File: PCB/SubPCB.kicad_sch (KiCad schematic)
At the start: 61 parts, among them U10 TLP222A, U11 TLP222A, U12 TLP222A, U13 TLP222A, U14 TLP222A, U15 TLP222A, U16 TLP222A, U17 TLP222A, U18 TLP222A, U2 TLP785, U3 TLP785, U38 MCP2562-E-P, U4 TLP785, U5 TLP785, U6 TLP785, U7 TLP785, U8 TLP785, U9 TLP785

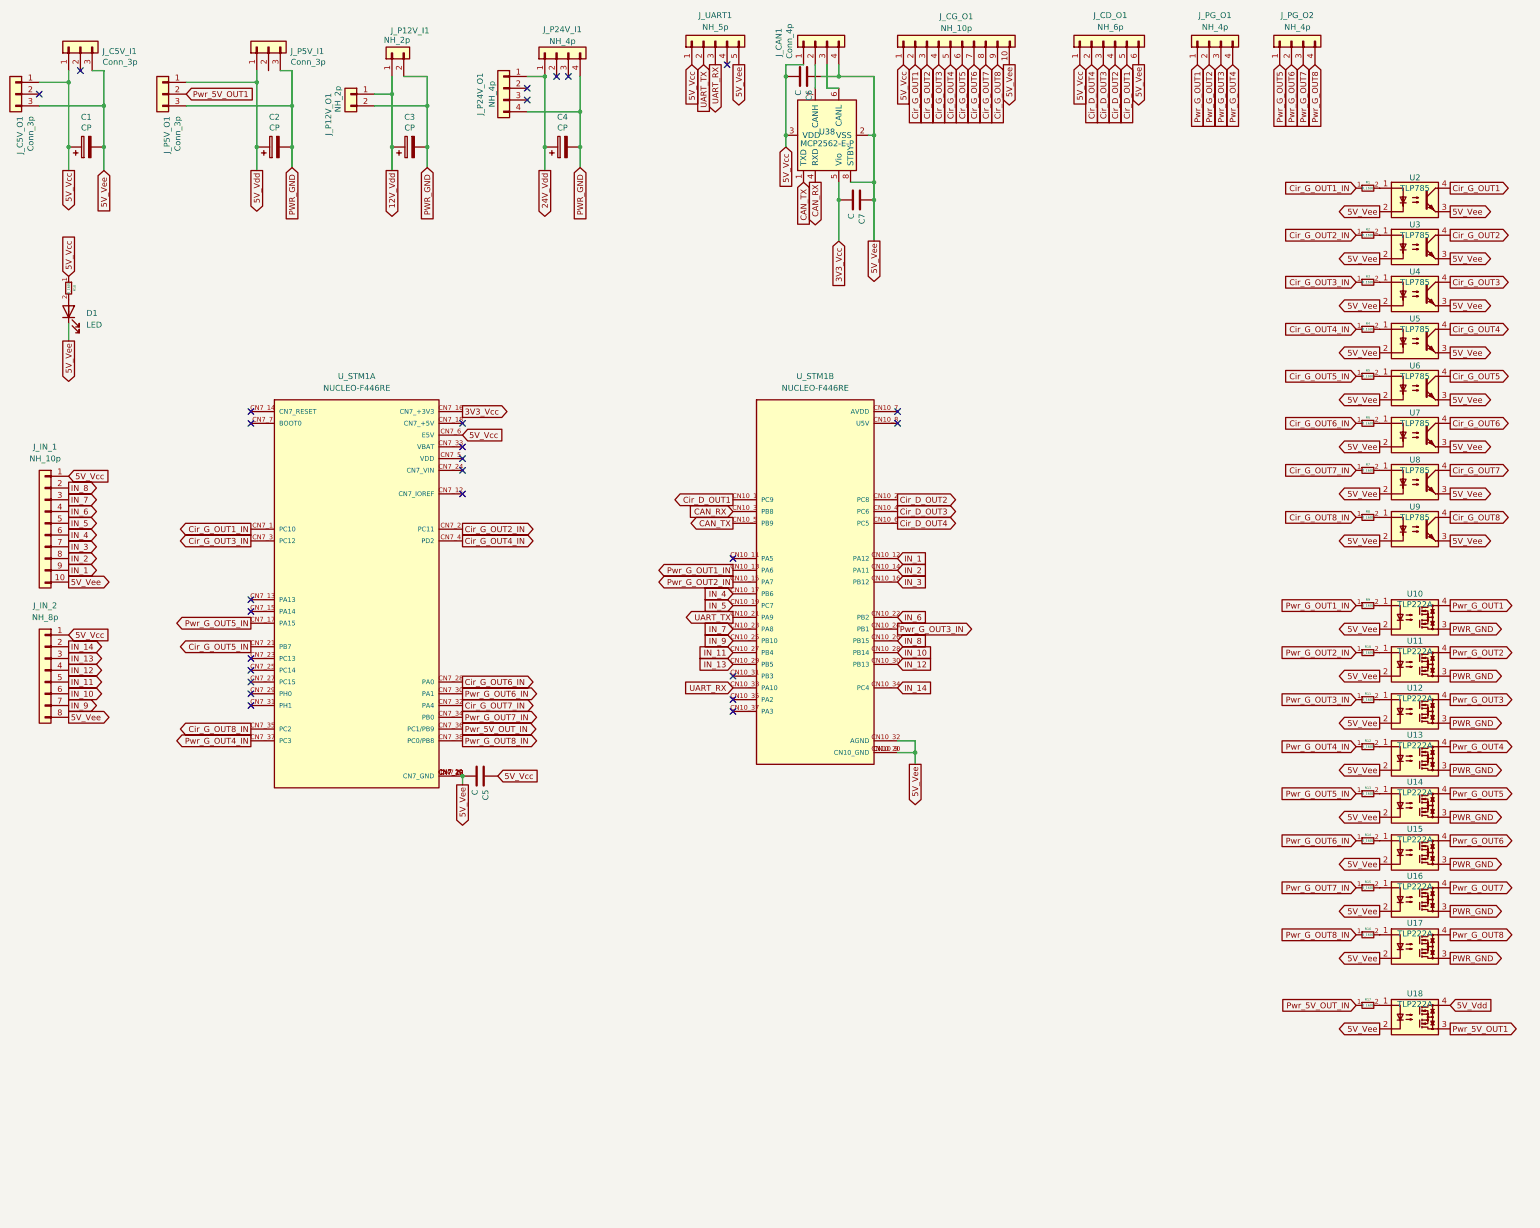
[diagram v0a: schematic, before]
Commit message: add
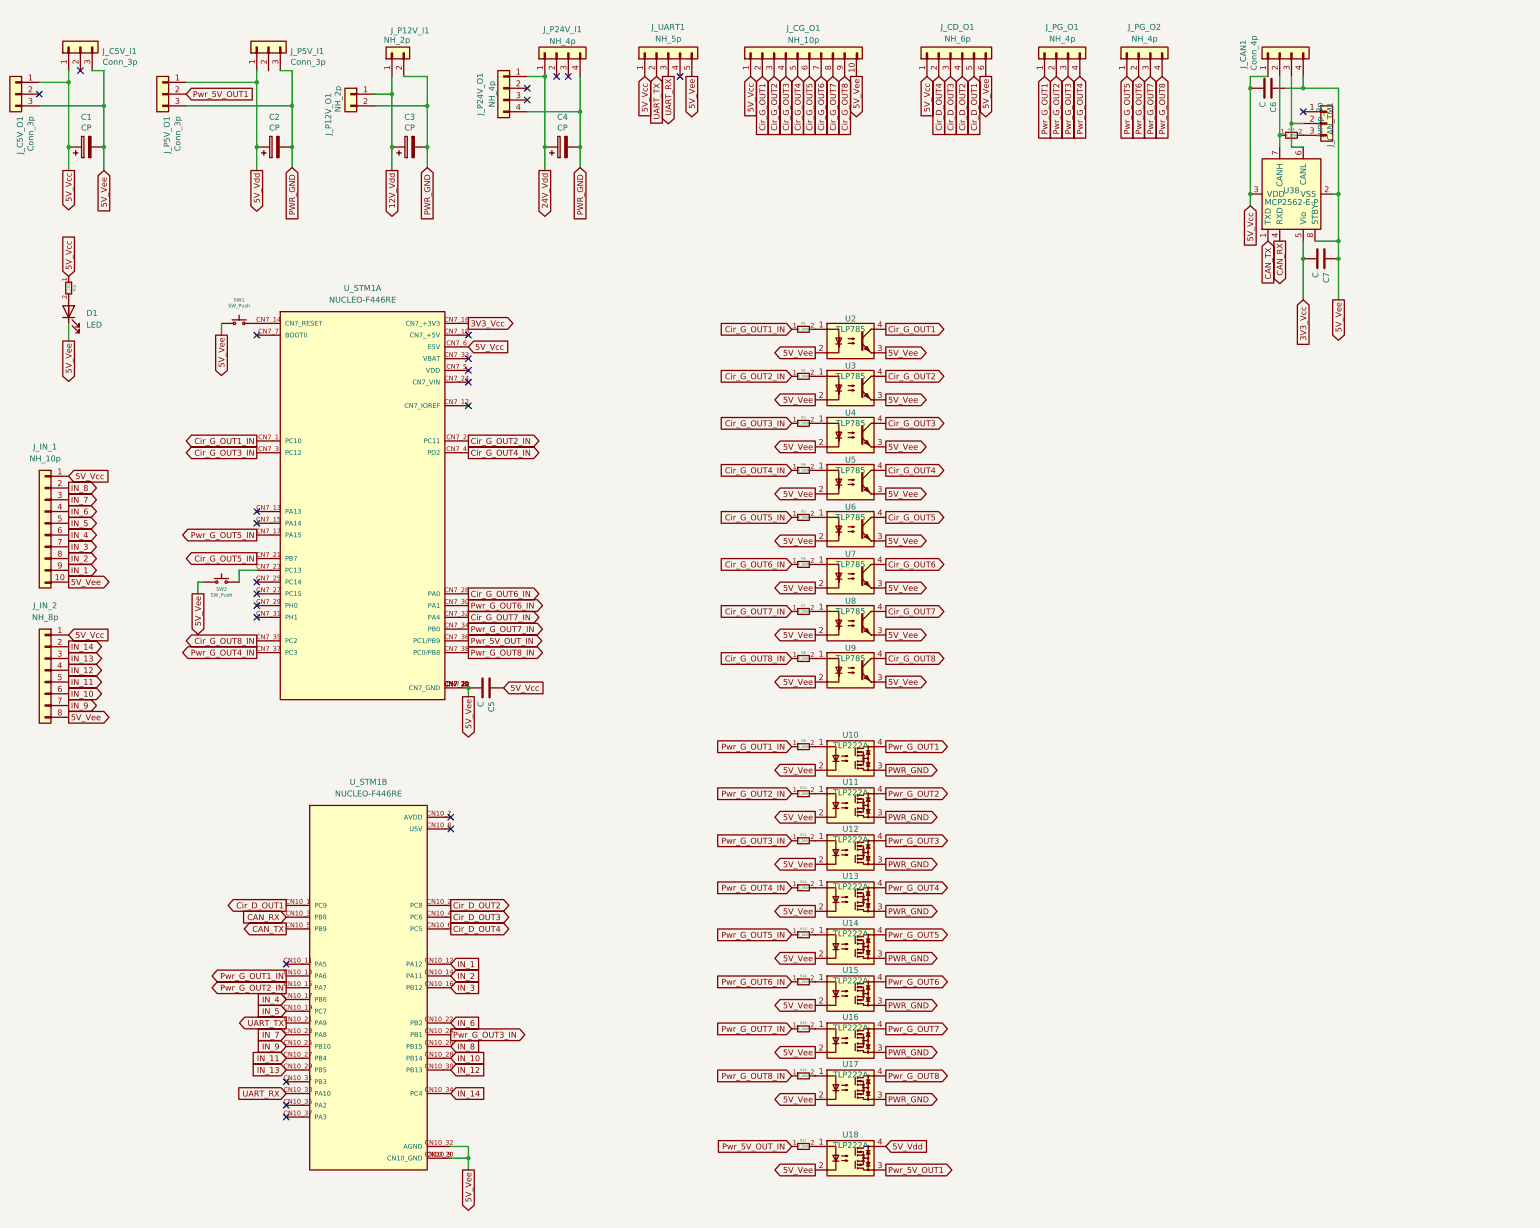
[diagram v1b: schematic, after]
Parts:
- added J_CAN_TM1: Jump_3p, KAZAAAN:Conn_3pin, symbol SubPCB-rescue:Conn_3p-KAZAAAN_Library
- added R19: R_1608, Resistor_SMD:R_0603_1608Metric_Pad0.98x0.95mm_HandSolder, symbol R_1608:R_1608
- added SW1, SW2: SW_Push, Button_Switch_THT:SW_PUSH_6mm_H5mm, symbol Switch:SW_Push
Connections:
- net 5V_Vee: now also SW1.1, SW2.1
- net at J_CAN1.2 (Pin_2), U38.7 (CANH): now also R19.1
- net at J_CAN1.3 (Pin_3), U38.6 (CANL): now also J_CAN_TM1.2 (Pin_2)
- net at U_STM1.CN7_14 (CN7_RESET): now also SW1.2
- net at U_STM1.CN7_23 (PC13): now also SW2.2
- new net: J_CAN_TM1.3 (Pin_3), R19.2
- no-connect marks 27 -> 26
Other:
- moved on the sheet: C5, C6, C7, J_CAN1, J_CD_O1, J_CG_O1, J_PG_O1, J_PG_O2, J_UART1, R1, R10, R11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
